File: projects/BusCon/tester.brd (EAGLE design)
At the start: 125.7 x 132.1 mm, 30 parts, among them IC1 74LS93N, IC10 74LS07N, IC11 74LS07N, IC12 74LS07N, IC13 74LS07N, IC14 74LS07N, IC15 74LS682N, IC16 74LS682N, IC17 74LS682N, IC18 74LS682N, IC19 74LS682N, IC2 74LS93N, IC20 74LS30N, IC21 74LS07N, IC22 74LS07N, IC23 74LS07N, IC24 74LS07N, IC25 74LS07N, IC26 74LS07N, IC3 74LS139N, IC4 74LS138N, IC5 74LS138N, IC6 74LS138N, IC7 74LS138N, IC8 74LS138N, IC9 74LS07N

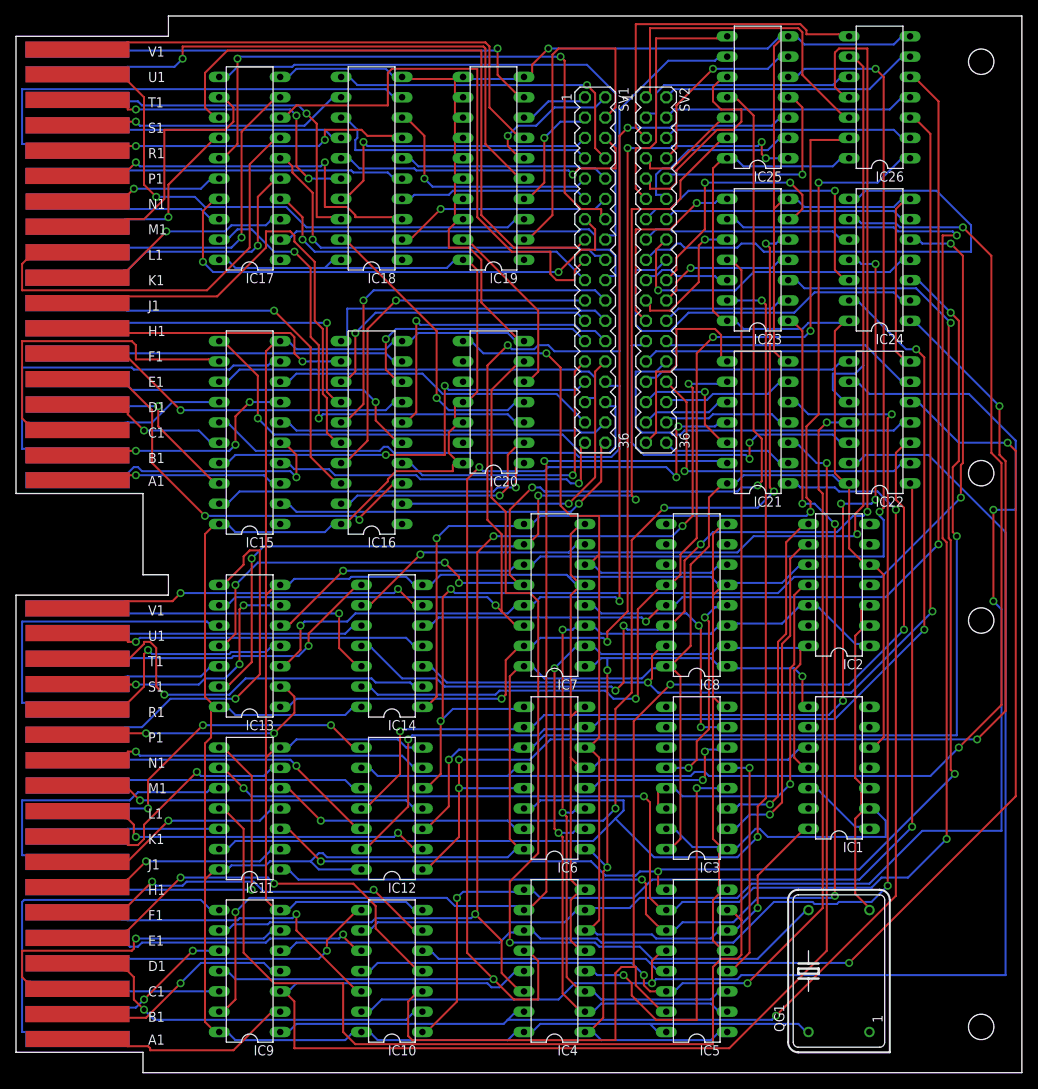
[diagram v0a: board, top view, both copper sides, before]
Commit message: Walk the project tree, making things pass current design rules.
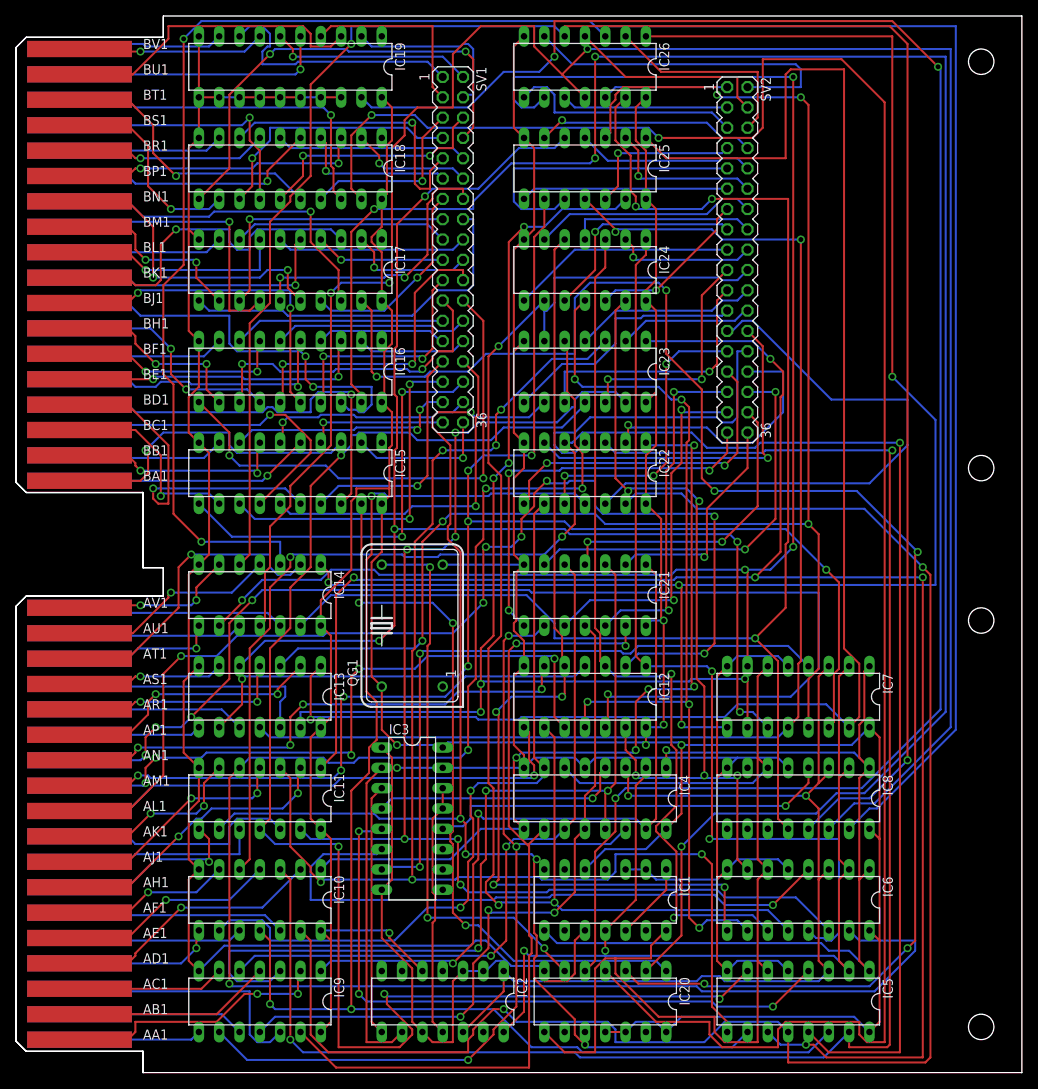
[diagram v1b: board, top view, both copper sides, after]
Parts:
- added U$2: OUTLINE-DOUBLE, dec-con:DOUBLE
- U$1: device dec-con:DOUBLE -> dec-con:EDGE-CON4
- moved IC20 76.2 mm to (73.7, 8.89), turned to 180 degrees
- moved IC2 71.9 mm to (53.3, 8.89), turned to 180 degrees
- moved QG1 68.6 mm to (49.5, 55.9)
- moved IC22 37.4 mm to (71.1, 74.9), turned to 180 degrees
- moved IC26 37.0 mm to (71.1, 125.7), turned to 180 degrees
- moved IC24 36.9 mm to (71.1, 100.3), turned to 180 degrees
- moved IC3 35.9 mm to (49.5, 31.8), turned to 270 degrees
- moved IC6 34.1 mm to (97.8, 21.6), turned to 180 degrees
- moved IC1 33.6 mm to (73.7, 21.6), turned to 180 degrees
- moved IC7 33.0 mm to (97.8, 47.0), turned to 180 degrees
- moved IC21 30.5 mm to (71.1, 59.7), turned to 180 degrees
- moved IC19 28.4 mm to (34.3, 125.7), turned to 180 degrees
- moved IC8 28.4 mm to (97.8, 34.3), turned to 180 degrees
- moved IC12 27.9 mm to (71.1, 47.0), turned to 180 degrees
- moved IC23 25.7 mm to (71.1, 87.6), turned to 180 degrees
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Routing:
- net OK2: track 28.2 -> 252.5 mm, vias 1 -> 4
- net OK4: track 36.9 -> 250.6 mm, vias 1 -> 2
- net OK5: track 22.8 -> 231.1 mm, vias 0 -> 3
- net GND: track 664.6 -> 506.8 mm
- net U1: track 138.1 -> 284.5 mm
- net OK3: track 59.3 -> 200.1 mm, vias 2 -> 6
- net V1: track 129.0 -> 250.8 mm
- net U2: track 151.6 -> 265.9 mm, vias 4 -> 3
- net AN2: track 39.1 -> 148.4 mm, vias 1 -> 5
- net VCC: track 534.1 -> 435.5 mm, vias 0 -> 6
- net AL1: track 45.8 -> 142.2 mm, vias 2 -> 7
- net K1: track 135.5 -> 220.8 mm, vias 5 -> 4
- net T1: track 124.6 -> 203.7 mm, vias 3 -> 4
- net F1: track 144.6 -> 222.1 mm, vias 2 -> 3
- net H1: track 151.7 -> 223.5 mm, vias 4 -> 5
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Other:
- outline, holes or cut-outs redrawn
